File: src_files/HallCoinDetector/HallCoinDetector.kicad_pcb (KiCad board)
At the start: 2 copper layers, 30.5 x 22.9 mm, 31 parts, among them M1 Motor_DC 3V, Q2 BSS214NW, SW1 On, U1 SE555D, U2 TPS61070, U3 49E Hall, U4 LM393

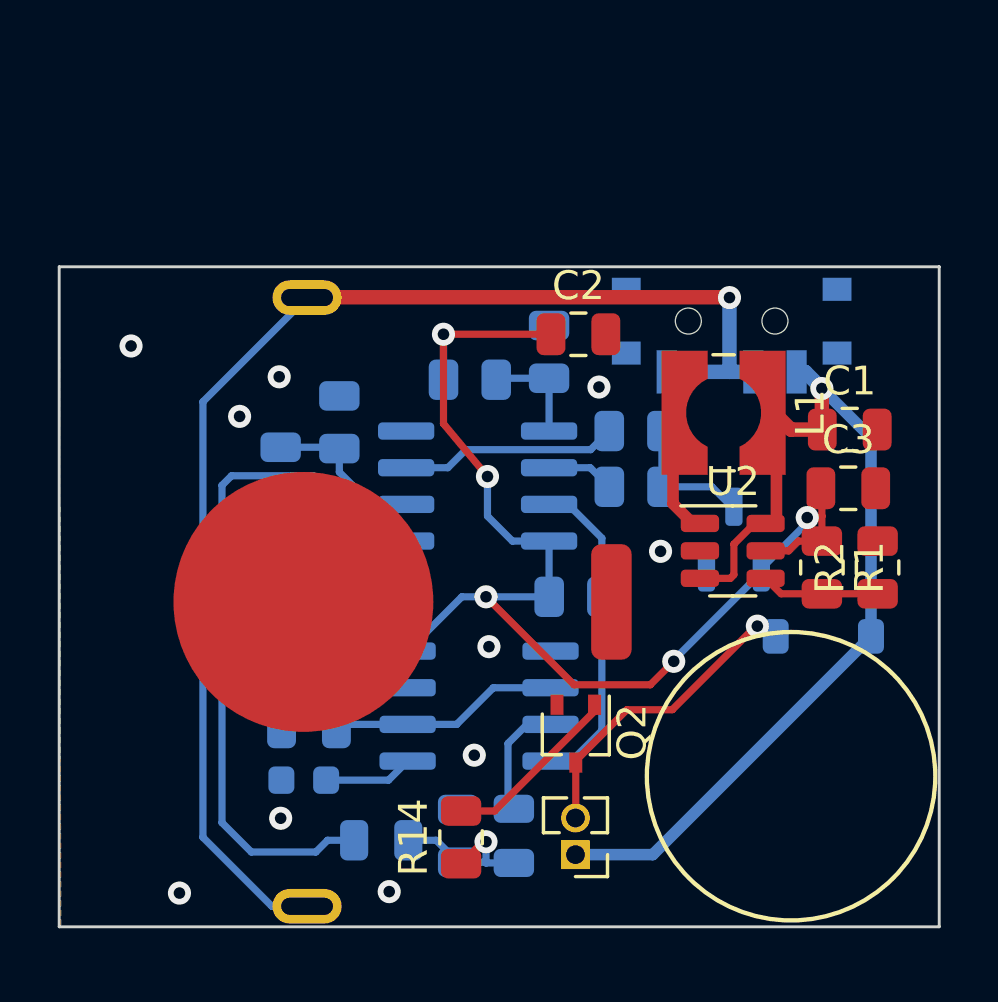
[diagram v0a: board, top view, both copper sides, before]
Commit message: panelizado
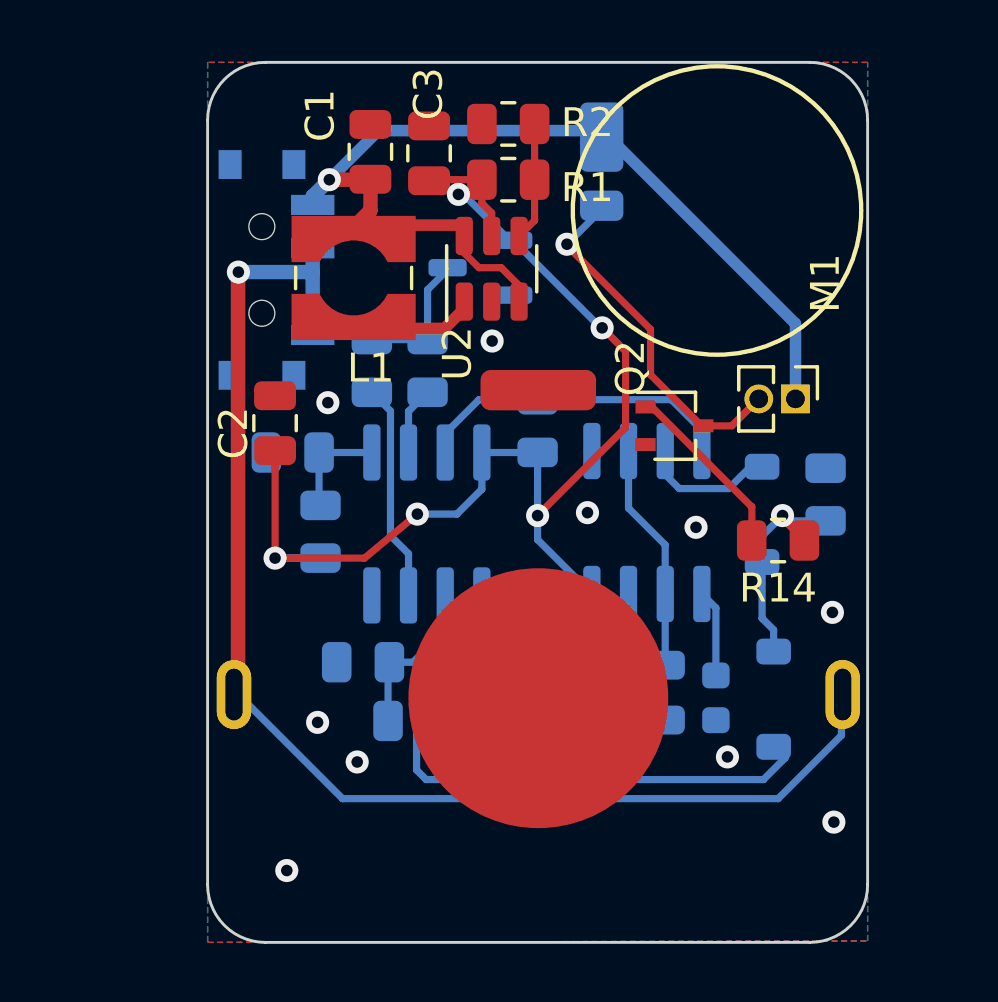
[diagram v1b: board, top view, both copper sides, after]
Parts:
- D1, D2: footprint Diode_SMD:D_0805_2012Metric -> Diode_SMD:D_SOD-123
- D3: footprint Diode_SMD:D_SOD-123 -> Diode_SMD:D_PowerDI-123
- R1, R13: value 1M -> 910k
- R2: value 110K -> 100k
- moved R2 20.0 mm to (165.4, 96.7), turned to 180 degrees
- moved C1 19.2 mm to (160.6, 97.6), turned to 90 degrees
- moved C3 18.6 mm to (162.7, 97.7), turned to 90 degrees
- moved D3 18.1 mm to (168.7, 98.0), turned to -90 degrees
- moved M1 17.5 mm to (175.4, 106.2), turned to -90 degrees
- moved R13 17.4 mm to (176.4, 109.5)
- moved R1 17.3 mm to (165.4, 98.6), turned to 0 degrees
- moved SW1 16.1 mm to (157.2, 101.7), turned to 90 degrees
- moved R14 15.0 mm to (174.8, 111.1), turned to 180 degrees
- moved C4 14.6 mm to (172.6, 116.5), turned to -90 degrees
- moved D1 14.4 mm to (174.6, 116.6), turned to -90 degrees
- moved D2 14.1 mm to (174.2, 110.2)
- moved L1 13.6 mm to (160.1, 102.0), turned to 0 degrees
- moved U3 12.9 mm to (164.4, 101.6), turned to 180 degrees
- moved U2 12.9 mm to (164.8, 101.7), turned to 90 degrees
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- renumbered r12 to R12
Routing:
- net Net-(D1-A): track 25.8 -> 21.9 mm
- net Net-(D3-A): track 10.3 -> 12.9 mm
- net Net-(D1-K): track 6.24 -> 8.26 mm
- net /3V: track 34.9 -> 34.3 mm
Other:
- board size 30.5 x 22.9 mm -> 22.9 x 30.5 mm
